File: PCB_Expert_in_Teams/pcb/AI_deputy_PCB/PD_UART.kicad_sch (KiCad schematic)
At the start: 31 parts, among them IC7 CYPD3177-24LQXQ, J16 USB_C_Receptacle_USB2.0_16P, Q2 DMP3098LSD-13, Q4 DMP3098LSD-13

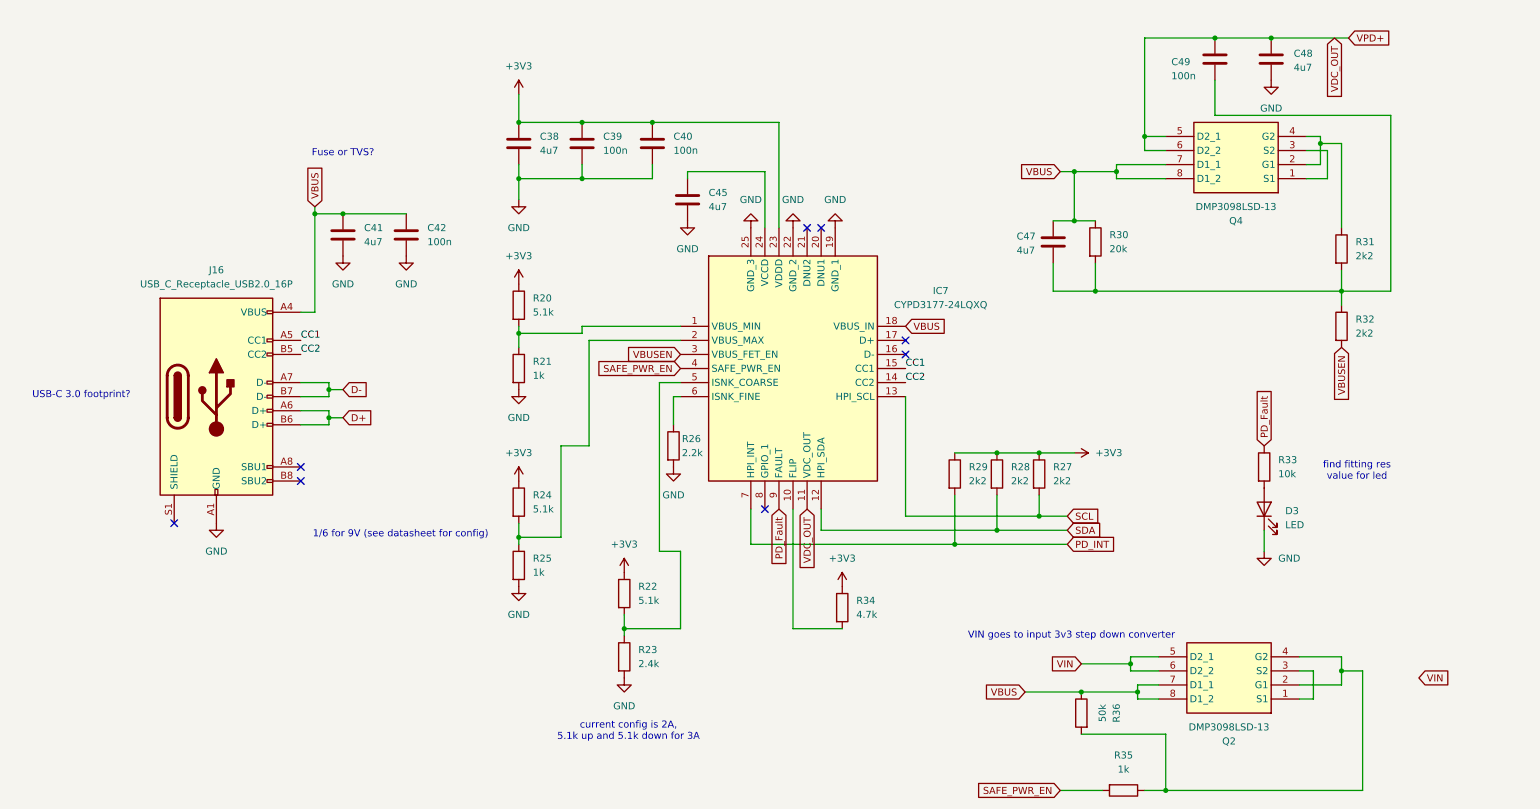
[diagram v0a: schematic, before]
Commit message: update schematic from desktop
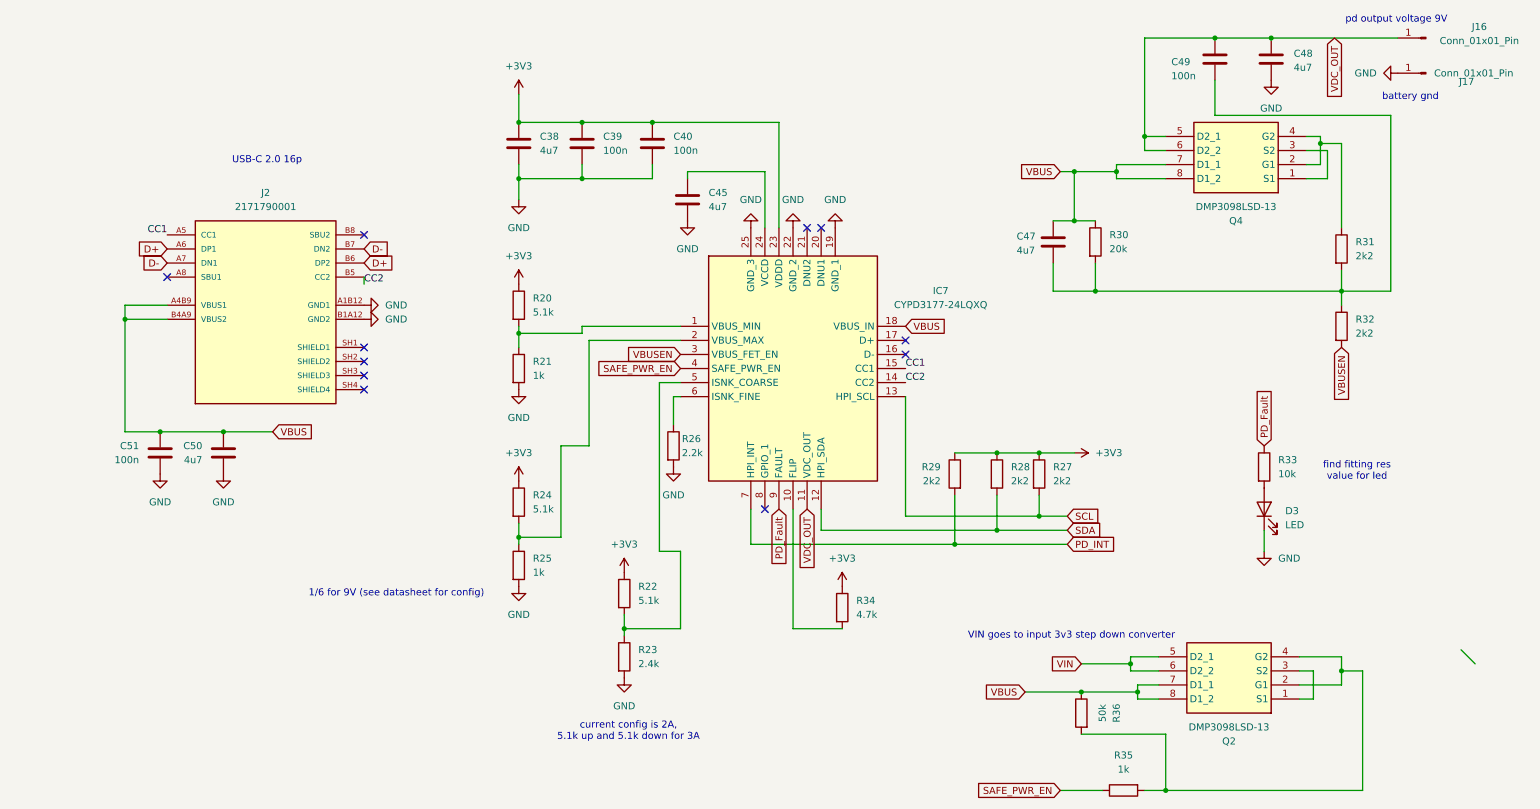
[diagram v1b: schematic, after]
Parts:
- removed C41: 4u7, Capacitor_SMD:C_0805_2012Metric_Pad1.18x1.45mm_HandSolder, symbol Device:C
- removed C42: 100n, Capacitor_SMD:C_0805_2012Metric_Pad1.18x1.45mm_HandSolder, symbol Device:C
- removed J16: USB_C_Receptacle_USB2.0_16P, EXT_AI_DEPUTY_Library:MOLEX_1054500101, symbol Connector:USB_C_Receptacle_USB2.0_16P
- added C50: 4u7, Capacitor_SMD:C_0805_2012Metric_Pad1.18x1.45mm_HandSolder, symbol Device:C
- added C51: 100n, Capacitor_SMD:C_0805_2012Metric_Pad1.18x1.45mm_HandSolder, symbol Device:C
- added J16, J17: Conn_01x01_Pin, TestPoint:TestPoint_Pad_4.0x4.0mm, symbol Connector:Conn_01x01_Pin
- added J2: 2171790001, EXT_AI_DEPUTY_Library:MOLEX_2171790001, symbol USBC-2.0-16p-molex-217179:2171790001
- C47: footprint (none) -> Capacitor_SMD:C_0805_2012Metric_Pad1.18x1.45mm_HandSolder
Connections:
- net CC1: now also J2.A5 (CC1)
- net CC2: now also J2.B5 (CC2)
- net D+: now also J2.A6 (DP1), J2.B6 (DP2)
- net D-: now also J2.A7 (DN1), J2.B7 (DN2)
- net GND: now also C50.2, C51.2, J17.1 (Pin_1), J2.A1B12 (GND1), J2.B1A12 (GND2)
- net SAFE_PWR_EN: now also R35.1; no longer R35.2
- net VBUS: now also C50.1, C51.1, J2.A4B9 (VBUS1), J2.B4A9 (VBUS2)
- net VDC_OUT: now also J16.1 (Pin_1)
- net at Q2.2 (G1), Q2.4 (G2), R36.2: now also R35.2; no longer R35.1
- no-connect marks 8 -> 11
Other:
- note added: "USB-C 2.0 16p"
- note added: "battery gnd"
- note added: "pd output voltage 9V"
- note removed: "Fuse or TVS?"
- note removed: "USB-C 3.0 footprint?"
- moved on the sheet: R35
